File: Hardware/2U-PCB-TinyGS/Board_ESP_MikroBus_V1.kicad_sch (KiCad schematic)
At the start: 15 parts, among them J1 Bus Standard, J1 Conn_01x19, J2 Conn_01x19, U1 ESP32-DEVKITC-32D

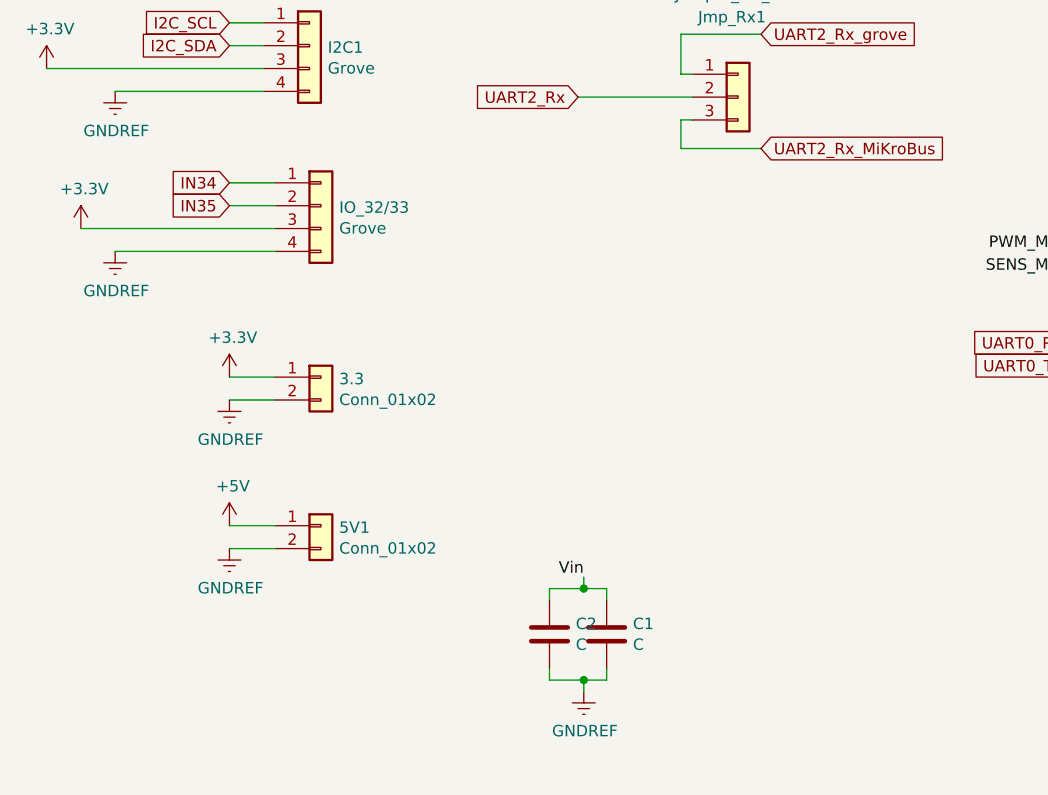
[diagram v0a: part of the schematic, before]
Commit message: Design changed
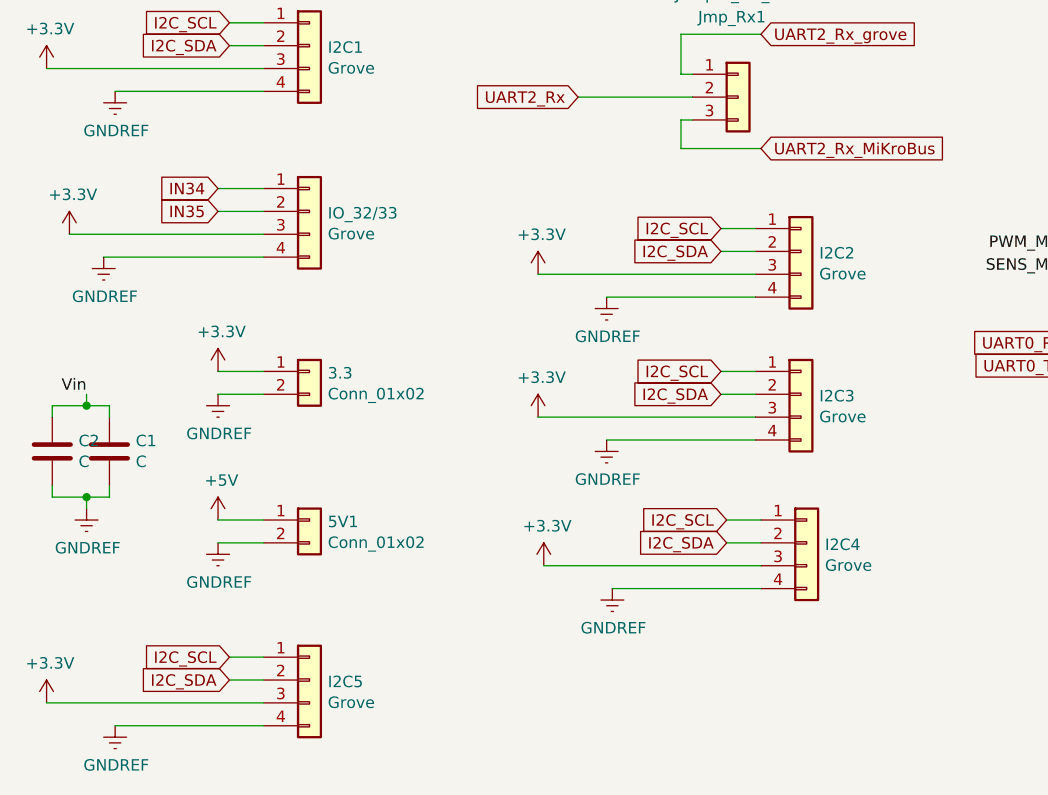
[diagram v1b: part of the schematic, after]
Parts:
- added I2C2, I2C3, I2C4, I2C5: Grove, Connector:NS-Tech_Grove_1x04_P2mm_Vertical, symbol Connector_Generic:Conn_01x04
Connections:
- net +3.3V: now also I2C2.3 (Pin_3), I2C3.3 (Pin_3), I2C4.3 (Pin_3), I2C5.3 (Pin_3)
- net GNDREF: now also I2C2.4 (Pin_4), I2C3.4 (Pin_4), I2C4.4 (Pin_4), I2C5.4 (Pin_4)
- net I2C_SCL: now also I2C2.1 (Pin_1), I2C3.1 (Pin_1), I2C4.1 (Pin_1), I2C5.1 (Pin_1)
- net I2C_SDA: now also I2C2.2 (Pin_2), I2C3.2 (Pin_2), I2C4.2 (Pin_2), I2C5.2 (Pin_2)
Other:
- moved on the sheet: 3.3, 5V1, C1, C2, IO_32/33
